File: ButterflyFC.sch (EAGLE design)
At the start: 7 parts

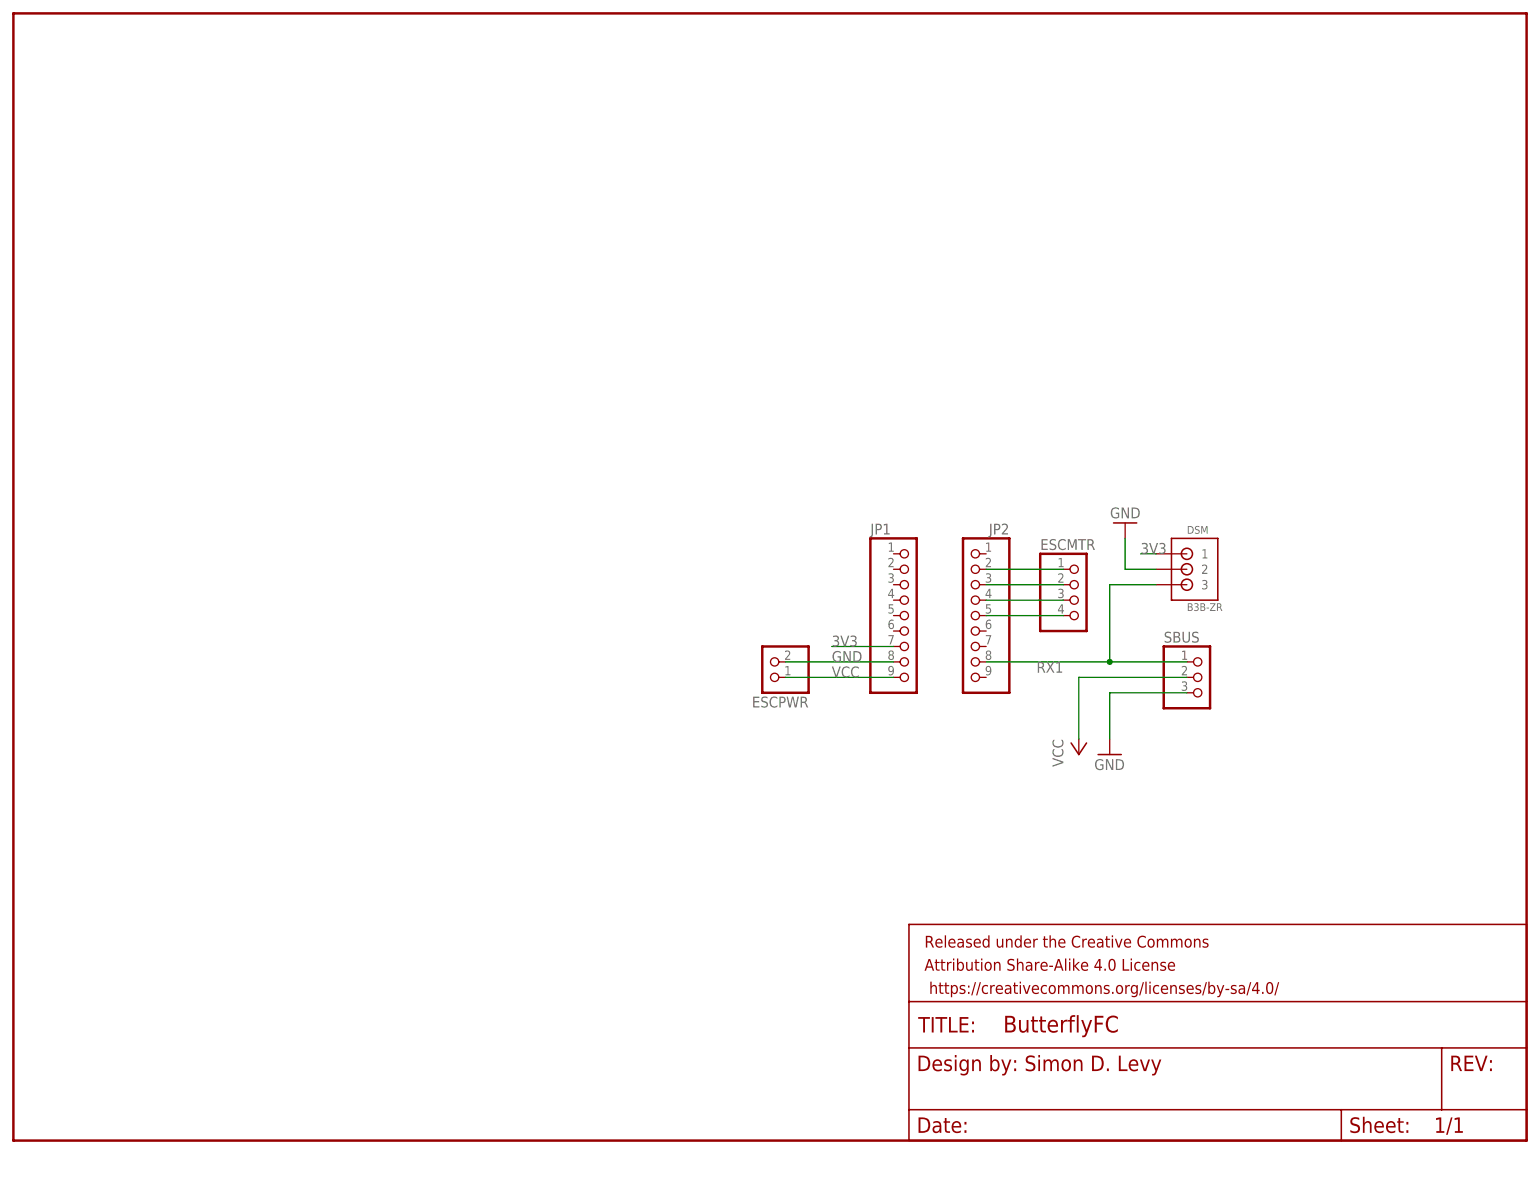
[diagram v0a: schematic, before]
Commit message: Rebuild board
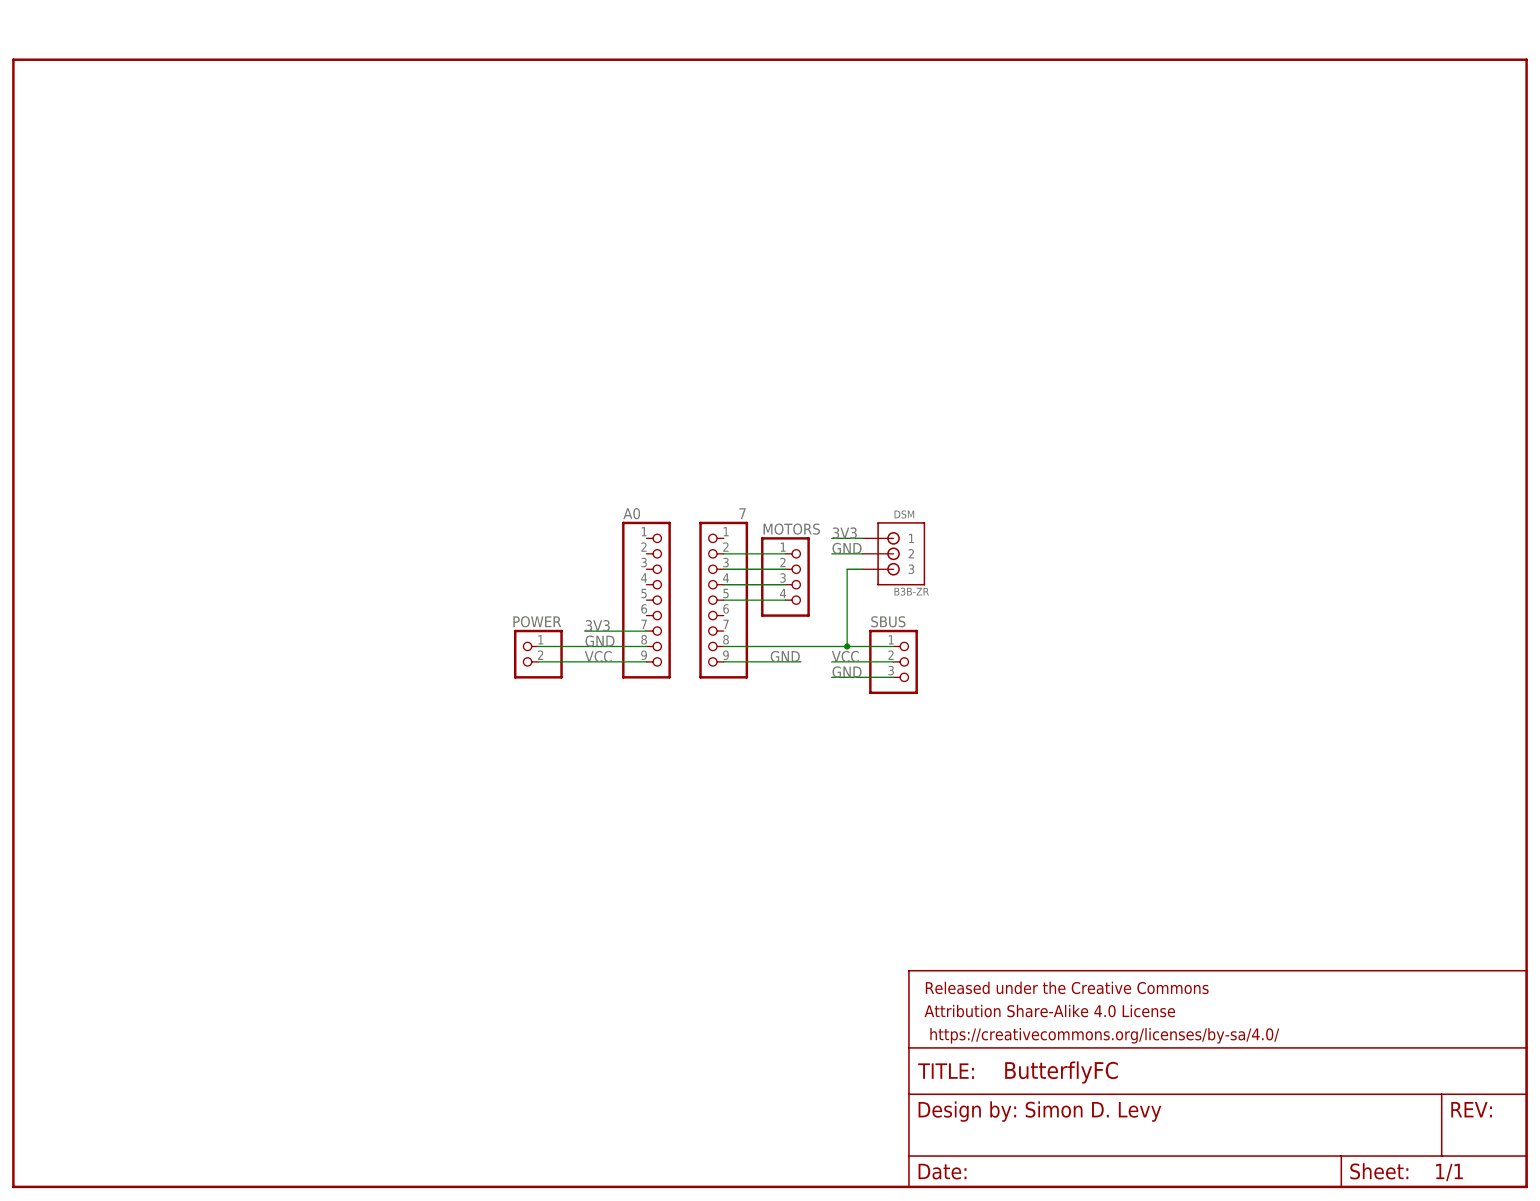
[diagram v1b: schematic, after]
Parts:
- removed ESCMTR: (no value), pinhead:PINHD-1X4
- removed ESCPWR: (no value), pinhead:PINHD-1X2
- removed JP1, JP2: (no value), pinhead:PINHD-1X9
- added 7, A0: (no value), pinhead:PINHD-1X9
- added MOTORS: (no value), pinhead:PINHD-1X4
- added POWER: (no value), pinhead:PINHD-1X2
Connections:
- removed net N$6: ESCMTR.3, JP2.4
- removed net RX1: DSM.3, JP2.8, SBUS.1
- new net N$1: 7.2, MOTORS.1
- new net N$5: 7.8, DSM.3, SBUS.1
- net 3V3: now also A0.7; no longer JP1.7
- net GND: now also 7.9, A0.8, POWER.1; no longer ESCPWR.2, JP1.8
- net N$2: now also 7.3, MOTORS.2; no longer ESCMTR.1, JP2.2
- net N$3: now also 7.4, MOTORS.3; no longer ESCMTR.4, JP2.5
- net N$4: now also 7.5, MOTORS.4; no longer ESCMTR.2, JP2.3
- net VCC: now also A0.9, POWER.2; no longer ESCPWR.1, JP1.9
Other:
- moved on the sheet: DSM, SBUS

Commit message: Re-routed board
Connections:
- net N$1 renamed M4
- net N$2 renamed M3
- net N$3 renamed M2
- net N$4 renamed M1
- net N$5 renamed RX1
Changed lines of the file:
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@@
 </segment>
 </net>
-<net name="N$1" class="0">
+<net name="M4" class="0">
 <segment>
 <pinref part="7" gate="A" pin="2"/>
@@
 </segment>
 </net>
-<net name="N$2" class="0">
+<net name="M3" class="0">
 <segment>
 <pinref part="7" gate="A" pin="3"/>
@@
 </segment>
 </net>
-<net name="N$3" class="0">
+<net name="M2" class="0">
 <segment>
 <pinref part="7" gate="A" pin="4"/>
@@
 </segment>
 </net>
-<net name="N$4" class="0">
+<net name="M1" class="0">
 <segment>
 <pinref part="7" gate="A" pin="5"/>
@@
 </segment>
 </net>
-<net name="N$5" class="0">
+<net name="RX1" class="0">
 <segment>
 <pinref part="7" gate="A" pin="8"/>
